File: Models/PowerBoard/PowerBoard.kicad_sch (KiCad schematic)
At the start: 0 parts

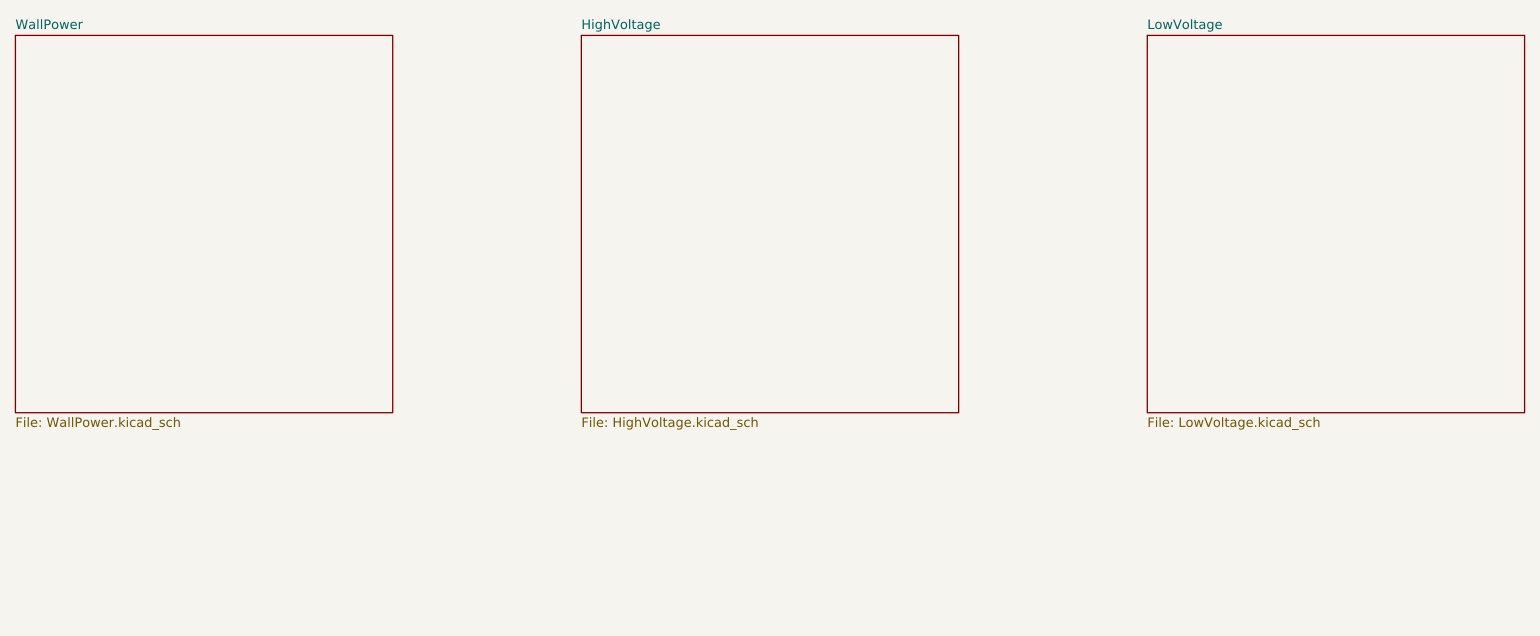
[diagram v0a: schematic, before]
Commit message: Save progress
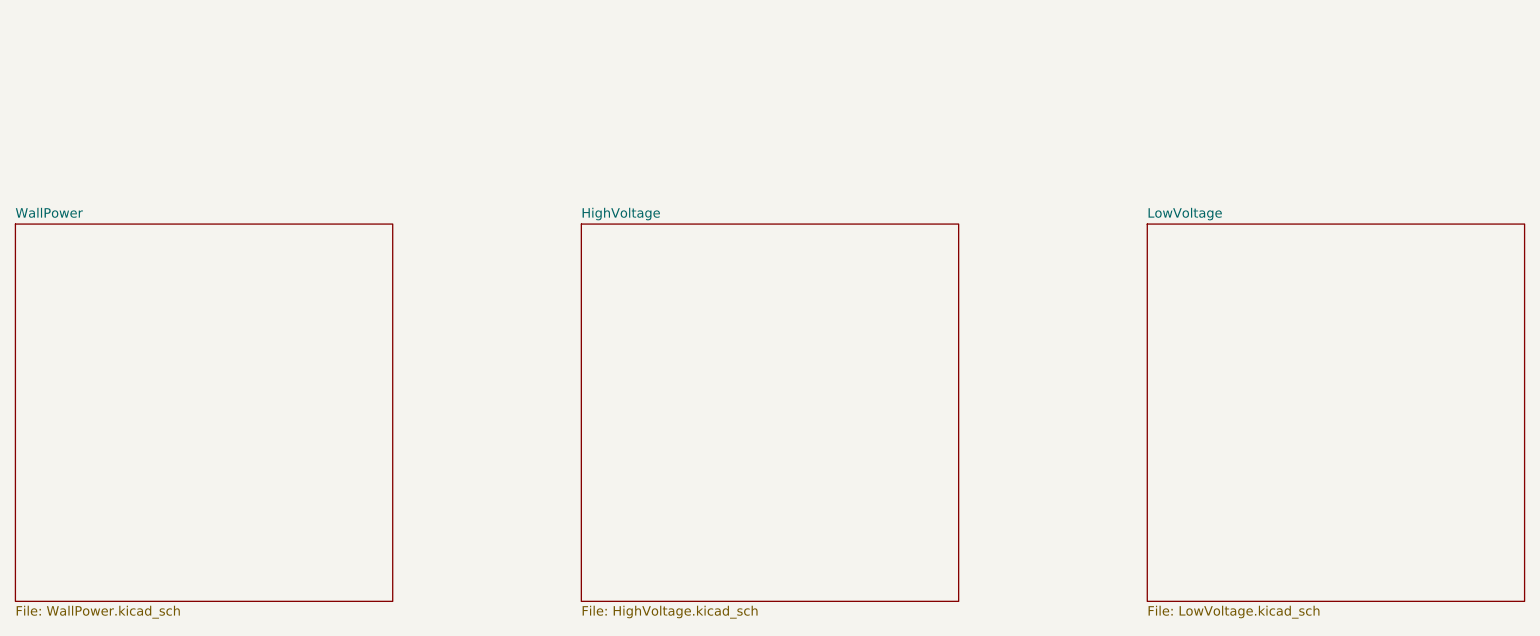
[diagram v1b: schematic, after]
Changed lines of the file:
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@@
 	(paper "A4")
 	(sheet
-		(at 50.8 50.8)
+		(at 50.8 76.2)
 		(size 50.8 50.8)
 		(exclude_from_sim no)
@@
 		)
 		(property "Sheetname" "WallPower"
-			(at 50.8 50.0884 0)
+			(at 50.8 75.4884 0)
 			(effects
 				(font
@@
 		)
 		(property "Sheetfile" "WallPower.kicad_sch"
-			(at 50.8 102.1846 0)
+			(at 50.8 127.5846 0)
 			(effects
 				(font
@@
 		)
 		(instances
-			(project "MainBoard"
-				(path "/600cc1cc-74ca-4bfc-97a0-b230eb3afbcd/d30698e6-a0ca-49f4-86ac-6bca70afd28d"
+			(project "PowerBoard"
+				(path "/c19e9b7b-7f36-470c-862a-1a648d3f14f6"
+					(page "2")
+				)
+			)
+		)
+	)
+	(sheet
+		(at 127 76.2)
+		(size 50.8 50.8)
+		(exclude_from_sim no)
+		(in_bom yes)
+		(on_board yes)
+		(dnp no)
+		(fields_autoplaced yes)
+		(stroke
+			(width 0.1524)
+			(type solid)
+		)
+		(fill
+			(color 0 0 0 0.0000)
+		)
+		(property "Sheetname" "HighVoltage"
+			(at 127 75.4884 0)
+			(effects
+				(font
+					(size 1.27 1.27)
+				)
+				(justify left bottom)
+			)
+		)
+		(property "Sheetfile" "HighVoltage.kicad_sch"
+			(at 127 127.5846 0)
+			(effects
+				(font
+					(size 1.27 1.27)
+				)
+				(justify left top)
+			)
+		)
+		(instances
+			(project "PowerBoard"
+				(path "/c19e9b7b-7f36-470c-862a-1a648d3f14f6"
 					(page "3")
 				)
@@
 	)
 	(sheet
-		(at 203.2 50.8)
+		(at 203.2 76.2)
 		(size 50.8 50.8)
 		(exclude_from_sim no)
@@
 		)
 		(property "Sheetname" "LowVoltage"
-			(at 203.2 50.0884 0)
+			(at 203.2 75.4884 0)
 			(effects
 				(font
@@
 		)
 		(property "Sheetfile" "LowVoltage.kicad_sch"
-			(at 203.2 102.1846 0)
+			(at 203.2 127.5846 0)
 			(effects
 				(font
@@
 		)
 		(instances
-			(project "MainBoard"
-				(path "/600cc1cc-74ca-4bfc-97a0-b230eb3afbcd/d30698e6-a0ca-49f4-86ac-6bca70afd28d"
-					(page "5")
-				)
-			)
-		)
-	)
-	(sheet
-		(at 127 50.8)
-		(size 50.8 50.8)
-		(exclude_from_sim no)
-		(in_bom yes)
-		(on_board yes)
-		(dnp no)
-		(fields_autoplaced yes)
-		(stroke
-			(width 0.1524)
-			(type solid)
-		)
-		(fill
-			(color 0 0 0 0.0000)
-		)
-		(property "Sheetname" "HighVoltage"
-			(at 127 50.0884 0)
-			(effects
-				(font
-					(size 1.27 1.27)
-				)
-				(justify left bottom)
-			)
-		)
-		(property "Sheetfile" "HighVoltage.kicad_sch"
-			(at 127 102.1846 0)
-			(effects
-				(font
-					(size 1.27 1.27)
-				)
-				(justify left top)
-			)
-		)
-		(instances
-			(project "MainBoard"
-				(path "/600cc1cc-74ca-4bfc-97a0-b230eb3afbcd/d30698e6-a0ca-49f4-86ac-6bca70afd28d"
+			(project "PowerBoard"
+				(path "/c19e9b7b-7f36-470c-862a-1a648d3f14f6"
 					(page "4")
 				)
@@
 		)
 	)
+	(sheet_instances
+		(path "/"
+			(page "1")
+		)
+	)
+	(embedded_fonts no)
 )
